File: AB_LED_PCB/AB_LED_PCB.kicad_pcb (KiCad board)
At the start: 2 copper layers, 49.1 x 21.4 mm, 16 parts, among them J1 Conn_01x03_Male

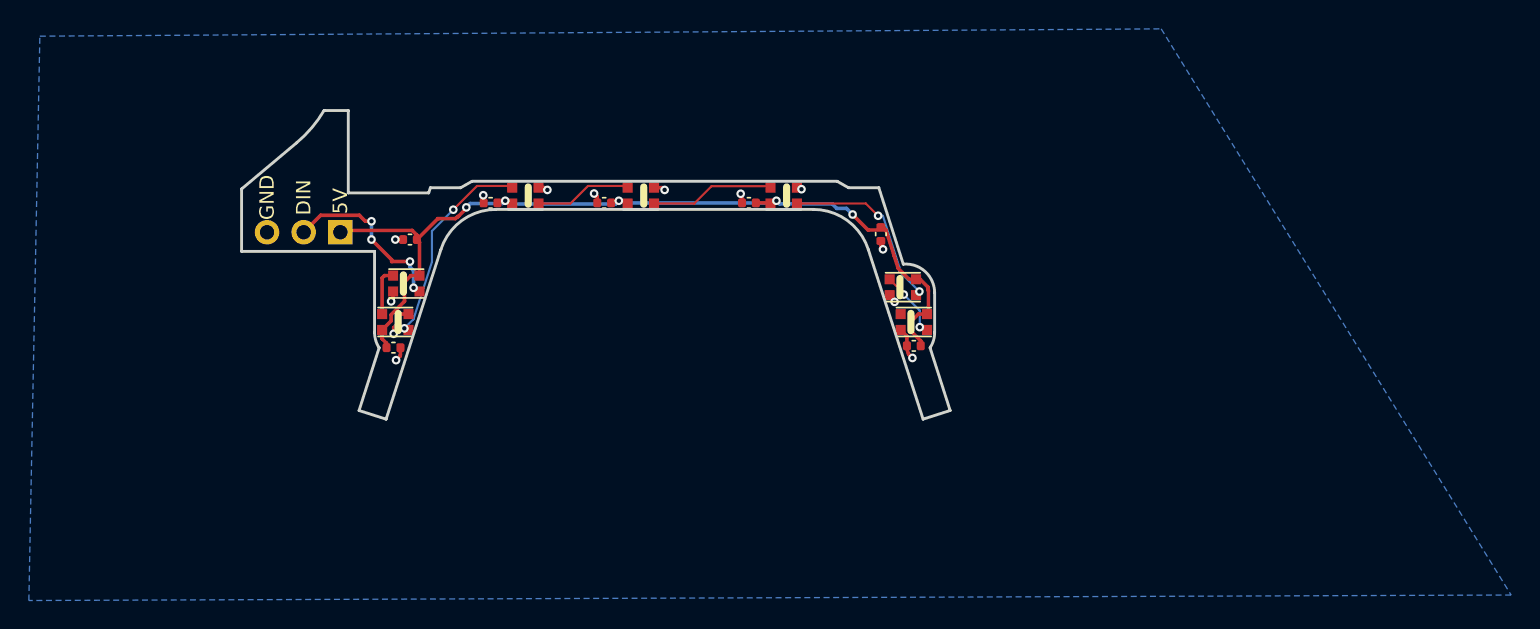
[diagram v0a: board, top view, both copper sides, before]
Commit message: fixed ercs
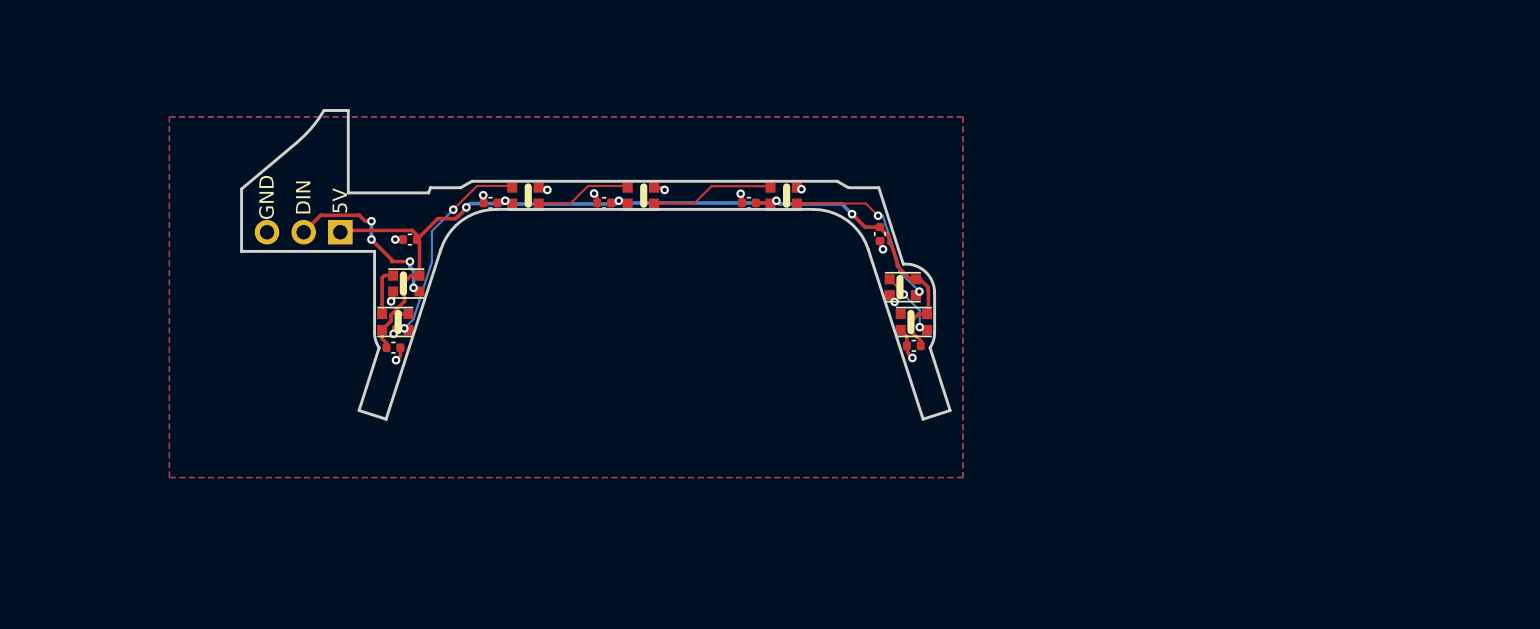
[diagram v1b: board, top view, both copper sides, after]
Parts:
- moved C4 0.06 mm to (194.2, 103.1)
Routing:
- added copper zone on F.Cu, net GND
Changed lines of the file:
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@@
     (thickness 1.6)
     (drawings 34)
-    (tracks 179)
+    (tracks 181)
     (zones 0)
     (modules 16)
@@
     (user_trace_width 0.15)
     (trace_clearance 0.15)
-    (zone_clearance 0.508)
+    (zone_clearance 0.25)
     (zone_45_only no)
     (trace_min 0.15)
@@
   )
   (module Capacitor_SMD:C_0402_1005Metric (layer F.Cu)
-    (at 194.31 103.124 270)
+    (at 194.2465 103.124 270)
     (descr "Capacitor SMD 0402 (1005 Metric), square (rectangular) end terminal, IPC_7351 nominal, (Body size source: IPC-SM-782 page 76, https://www.pcb-3d.com/wordpress/wp-content/uploads/ipc-sm-782a_amendment_1_and_2.pdf), generated with kicad-footprint-generator")
     (tags capacitor)
@@
   (segment (start 197.574432 106.850733) (end 197.557217 106.782293) (width 0.25) (layer F.Cu) (net 2))
   (segment (start 197.031924 106.257) (end 196.749 106.257) (width 0.25) (layer F.Cu) (net 2))
-  (segment (start 196.749 106.257) (end 196.265693 106.257) (width 0.25) (layer F.Cu) (net 2))
-  (segment (start 196.265693 106.257) (end 195.514072 105.505379) (width 0.25) (layer F.Cu) (net 2))
-  (segment (start 195.514072 105.505379) (end 195.242817 104.657999) (width 0.25) (layer F.Cu) (net 2))
-  (segment (start 194.660788 102.839788) (end 194.564 102.743) (width 0.25) (layer F.Cu) (net 2))
-  (segment (start 195.242817 104.657999) (end 194.660788 102.839788) (width 0.25) (layer F.Cu) (net 2))
   (segment (start 162.151 103.195) (end 162.151 103.505) (width 0.25) (layer F.Cu) (net 2))
   (segment (start 161.82599 102.86999) (end 162.151 103.195) (width 0.25) (layer F.Cu) (net 2))
@@
   (segment (start 187.071 100.81435) (end 186.916849 100.968501) (width 0.25) (layer B.Cu) (net 2))
   (segment (start 176.727415 100.968501) (end 176.573264 100.81435) (width 0.25) (layer B.Cu) (net 2))
-  (segment (start 194.660788 102.839788) (end 193.424024 102.839788) (width 0.25) (layer F.Cu) (net 2))
-  (segment (start 193.424024 102.839788) (end 192.352745 101.768509) (width 0.25) (layer F.Cu) (net 2))
-  (via (at 192.352745 101.768509) (size 0.6) (drill 0.3) (layers F.Cu B.Cu) (net 2))
-  (segment (start 191.252856 101.346) (end 191.930236 101.346) (width 0.25) (layer B.Cu) (net 2))
-  (segment (start 191.930236 101.346) (end 192.352745 101.768509) (width 0.25) (layer B.Cu) (net 2))
-  (segment (start 191.252856 101.346) (end 190.935356 101.0285) (width 0.25) (layer B.Cu) (net 2))
+  (via (at 192.316578 101.741269) (size 0.6) (drill 0.3) (layers F.Cu B.Cu) (net 2))
+  (segment (start 193.219309 102.644) (end 192.316578 101.741269) (width 0.25) (layer F.Cu) (net 2))
+  (segment (start 194.31 102.644) (end 193.219309 102.644) (width 0.25) (layer F.Cu) (net 2))
   (segment (start 187.28515 101.0285) (end 187.071 100.81435) (width 0.25) (layer B.Cu) (net 2))
-  (segment (start 190.935356 101.0285) (end 187.28515 101.0285) (width 0.25) (layer B.Cu) (net 2))
+  (segment (start 191.603809 101.0285) (end 187.28515 101.0285) (width 0.25) (layer B.Cu) (net 2))
+  (segment (start 192.316578 101.741269) (end 191.603809 101.0285) (width 0.25) (layer B.Cu) (net 2))
+  (segment (start 194.2465 102.644) (end 194.2465 102.6795) (width 0.25) (layer F.Cu) (net 2))
+  (segment (start 194.857595 103.290595) (end 194.8815 103.365275) (width 0.25) (layer F.Cu) (net 2))
+  (segment (start 194.2465 102.6795) (end 194.857595 103.290595) (width 0.25) (layer F.Cu) (net 2))
+  (segment (start 194.8815 103.365275) (end 194.8815 103.759) (width 0.25) (layer F.Cu) (net 2))
+  (segment (start 195.066878 103.944378) (end 195.453 105.150594) (width 0.25) (layer F.Cu) (net 2))
+  (segment (start 194.8815 103.759) (end 195.066878 103.944378) (width 0.25) (layer F.Cu) (net 2))
+  (segment (start 195.453 105.345202) (end 196.364798 106.257) (width 0.25) (layer F.Cu) (net 2))
+  (segment (start 196.364798 106.257) (end 196.749 106.257) (width 0.25) (layer F.Cu) (net 2))
+  (segment (start 195.453 105.150594) (end 195.453 105.345202) (width 0.25) (layer F.Cu) (net 2))
   (segment (start 170.587 101.007) (end 172.789992 101.007) (width 0.15) (layer F.Cu) (net 3))
   (segment (start 172.789992 101.007) (end 174.007633 99.789359) (width 0.15) (layer F.Cu) (net 3))
@@
     (polygon
       (pts
-        (xy 237.998 128.143) (xy 135.255 128.524) (xy 136.017 89.408) (xy 213.741 88.9)
+        (xy 200 120) (xy 145 120) (xy 145 95) (xy 200 95)
       )
     )
+  )
+  (zone (net 1) (net_name GND) (layer F.Cu) (hatch edge 0.508)
+    (connect_pads (clearance 0.25))
+    (min_thickness 0.2)
+    (fill yes (arc_segments 32) (thermal_gap 0.25) (thermal_bridge_width 0.25))
+    (polygon
+      (pts
+        (xy 200 120) (xy 145 120) (xy 145 95) (xy 200 95)
+      )
+    )
